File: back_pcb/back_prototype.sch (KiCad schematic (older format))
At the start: 66 parts, among them P5 CONN_01X04, P6 ATMEGA_HEADER, U1 PI ZERO

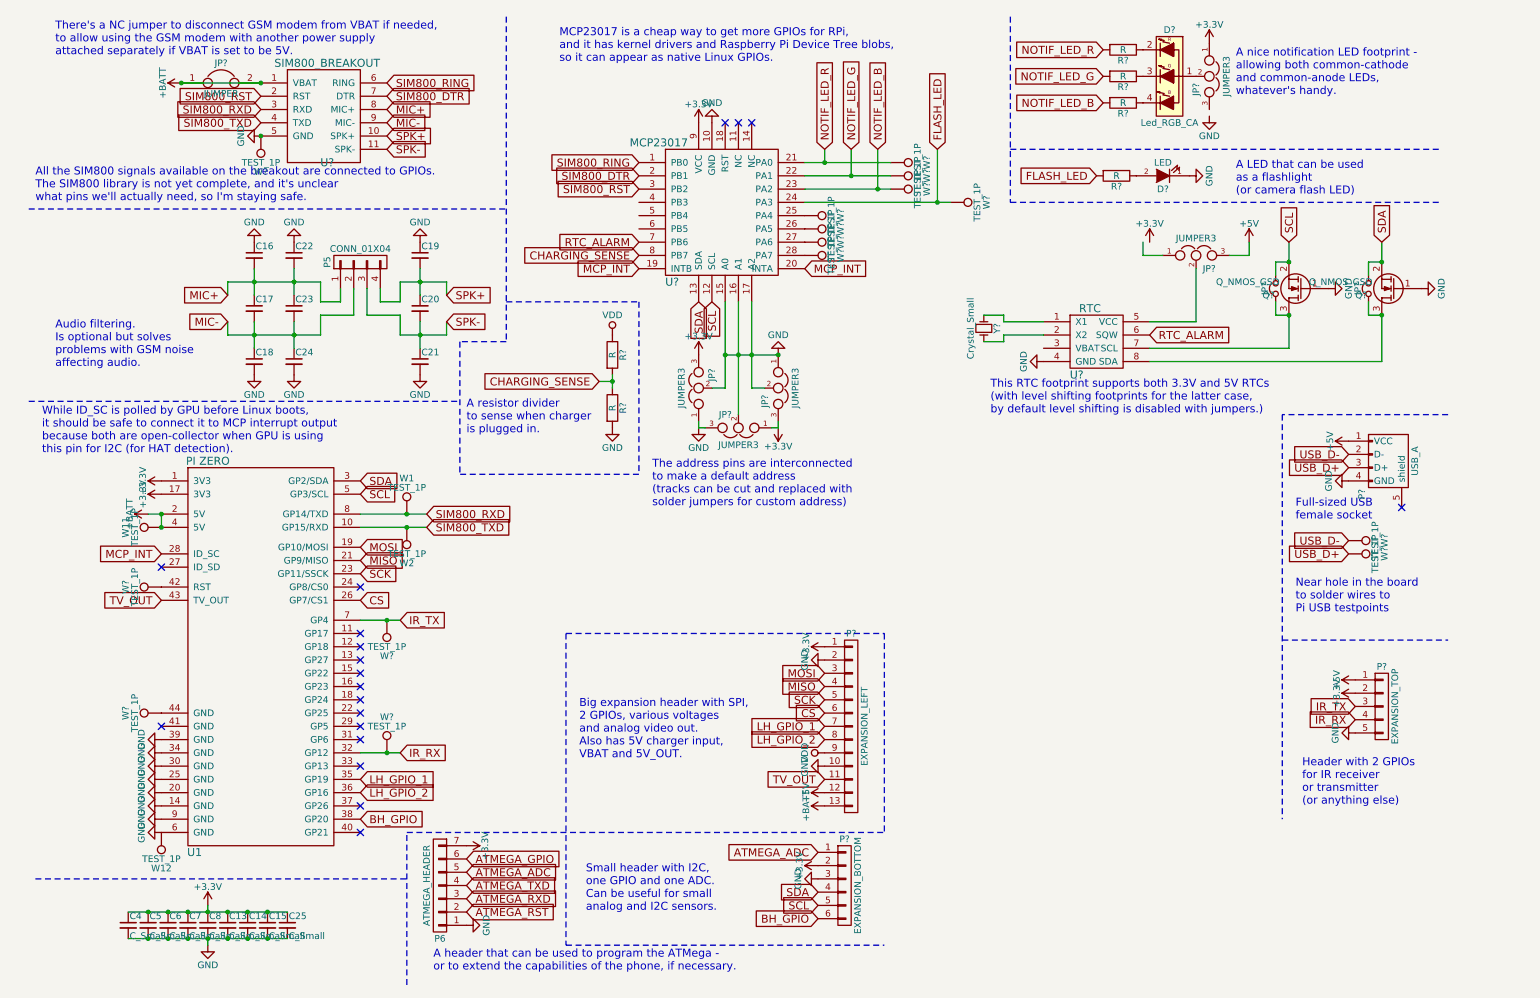
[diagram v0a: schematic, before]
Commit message: Beautiful annotations
So fabulous
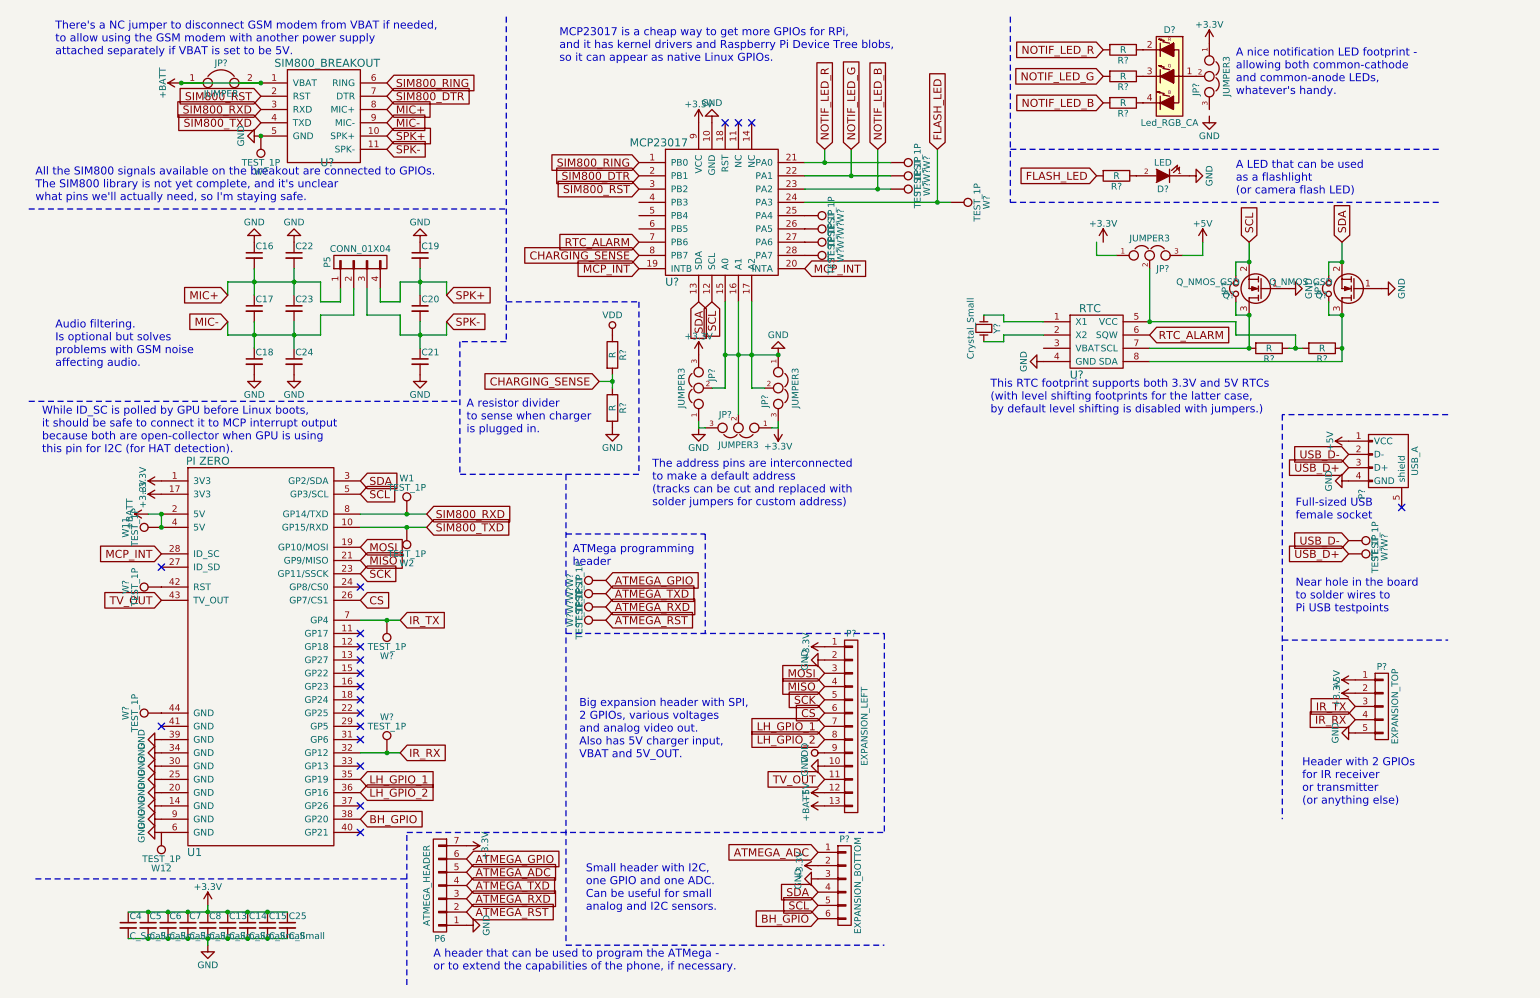
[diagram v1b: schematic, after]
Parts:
- added R? (x2): R, symbol R
- added W? (x4): TEST_1P, Measurement_Points:Measurement_Point_Square-SMD-Pad_Small, symbol TEST_1P
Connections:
- net ATMEGA_GPIO: now also W?.1
- net ATMEGA_RST: now also W?.1
- net ATMEGA_RXD: now also W?.1
- net ATMEGA_TXD: now also W?.1
- net at JP?.2, U?.5 (VCC): now also R?.1, R?.2
- net at JP?.1, Q?.3 (D), U?.7 (SCL): now also R?.2
- net at JP?.1, Q?.3 (D), U?.8 (SDA): now also R?.1
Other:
- note added: "ATMega programming \nheader"
- moved on the sheet: JP?, Q?

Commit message: Back board almost finished
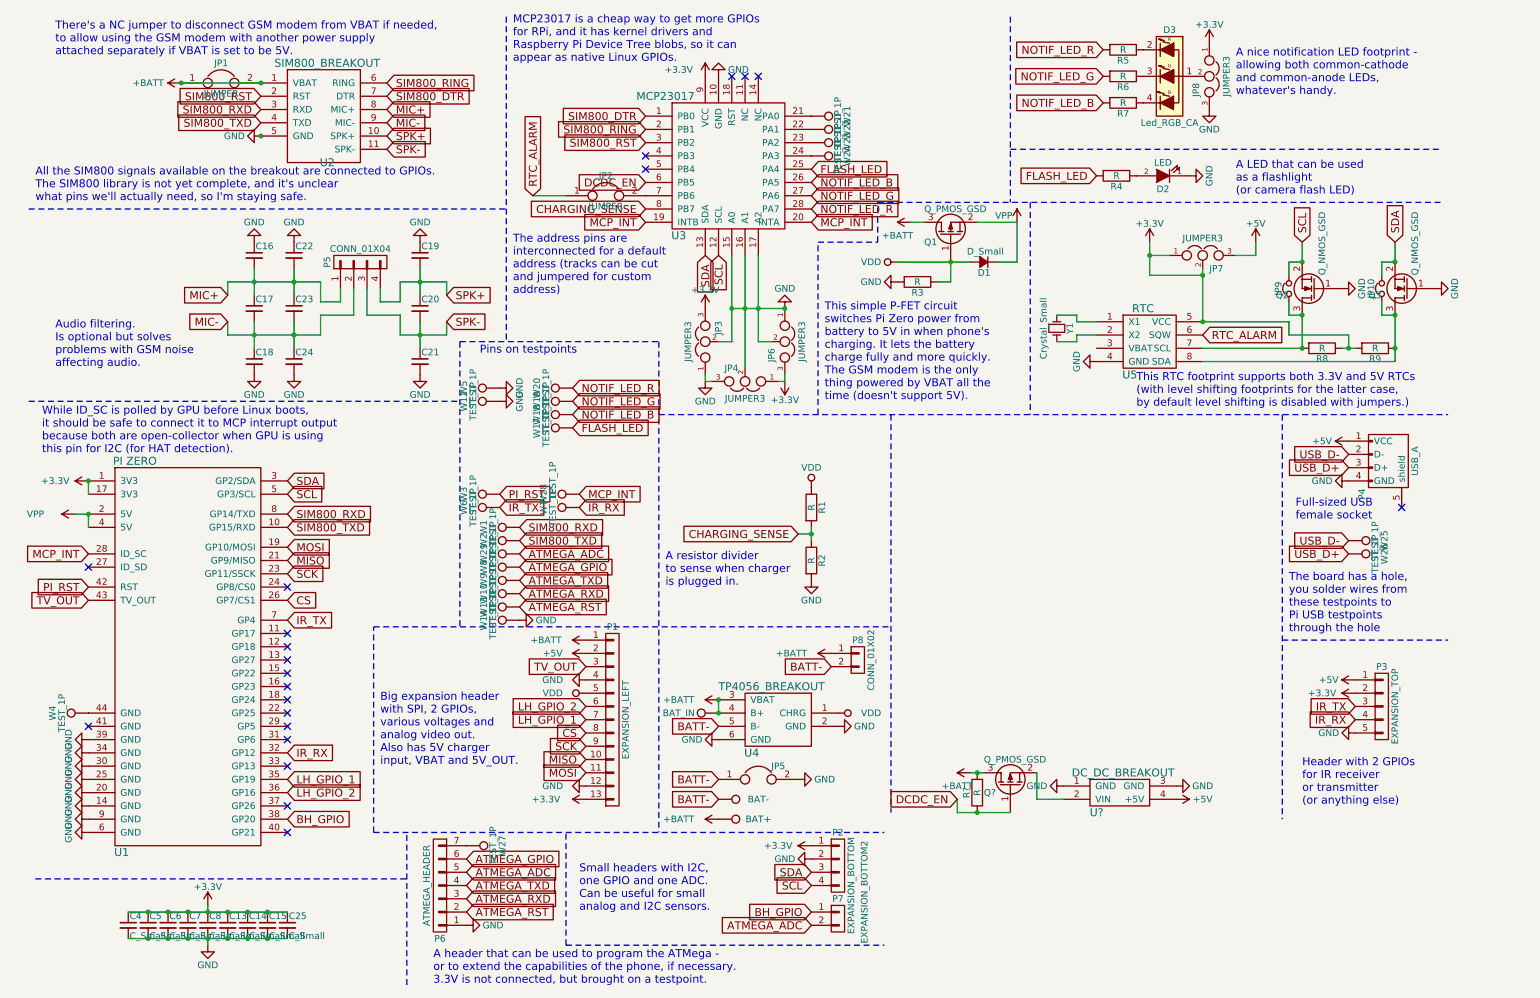
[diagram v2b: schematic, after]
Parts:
- removed P?: EXPANSION_BOTTOM, symbol CONN_01X06
- added D1: D_Small, Diodes_SMD:D_MiniMELF_Handsoldering, symbol D_Small
- added JP1, JP5: JUMPER, Connect:GS2, symbol JUMPER
- added P2: EXPANSION_BOTTOM, Pin_Headers:Pin_Header_Angled_1x04_Pitch2.54mm, symbol CONN_01X04
- added P7: EXPANSION_BOTTOM2, Pin_Headers:Pin_Header_Angled_1x02_Pitch2.54mm, symbol CONN_01X02
- added P8: CONN_01X02, footprints:JST_PH_S2B-PH-SM4-TB_02x2.00mm_Angled, symbol CONN_01X02
- added Q1, Q?: Q_PMOS_GSD, TO_SOT_Packages_SMD:SOT-23_Handsoldering, symbol Q_PMOS_GSD
- added R3, R?: R, Resistors_SMD:R_0805_HandSoldering, symbol R
- added U4: TP4056_BREAKOUT, footprints:TP4056_BREAKOUT, symbol TP4056_BREAKOUT
- added U?: DC_DC_BREAKOUT, symbol DC_DC_BREAKOUT
- added W14, W27, W28, W29: TEST_1P, Measurement_Points:Measurement_Point_Square-SMD-Pad_Small, symbol TEST_1P
- added W15: BAT-, Measurement_Points:Measurement_Point_Square-SMD-Pad_Small, symbol TEST_1P
- added W16: BAT+, Measurement_Points:Measurement_Point_Square-SMD-Pad_Small, symbol TEST_1P
- JP10, JP2, JP9: renamed from JP?; footprint (none) -> Connect:GS2
- JP3, JP4, JP6, JP7, JP8: renamed from JP?; footprint (none) -> Connect:GS3
- P1: renamed from P?; footprint (none) -> Pin_Headers:Pin_Header_Angled_1x13_Pitch2.54mm
- P3: renamed from P?; footprint (none) -> Pin_Headers:Pin_Header_Angled_1x05_Pitch2.54mm
- P4: renamed from P?; footprint (none) -> Connect:USB_A
- Q2, Q3: renamed from Q?; footprint (none) -> TO_SOT_Packages_SMD:SOT-23_Handsoldering
- R1, R2, R4, R5, R6, R7, R8, R9: renamed from R?; footprint (none) -> Resistors_SMD:R_0805_HandSoldering
- U2: renamed from U?; footprint (none) -> footprints:SIM800_BREAKOUT
- U3: renamed from U?; footprint (none) -> SMD_Packages:SOIC-28
- U5: renamed from U?; footprint (none) -> Housings_SOIC:SOIC-8_3.9x4.9mm_Pitch1.27mm
- W11: value TEST_1P -> BAT_IN
- Y1: renamed from Y?; footprint (none) -> Crystals:Crystal_SMD_G8-2pin_3.2x1.5mm_HandSoldering
- gave numbers to parts that had none: 21
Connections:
- net +3V3: now also JP7.1, JP7.2, P1.13 (P13), R8.1, R9.2, U5.5 (VCC), P2.1 (P1); no longer P1.1 (P1), P6.7 (P7)
- net +5V: now also P1.2 (P2), U?.4 (+5V); no longer P1.12 (P12)
- net +BATT: now also P1.1 (P1), JP1.1, JP1.2, P8.1 (P1), Q1.3 (D), Q?.3 (D), R?.2, U4.3 (VBAT), U4.4 (B+), W16.1; no longer JP2.1, JP2.2, P1.13 (P13), U1.2 (5V), U1.4 (5V)
- net ATMEGA_ADC: now also P7.2 (P2), W29.1
- net BH_GPIO: now also P7.1 (P1)
- net CS: now also P1.8 (P8); no longer P1.6 (P6)
- net FLASH_LED: now also U3.25 (PA4), W17.1; no longer U3.24 (PA3), W24.1
- net GND: now also JP8.3, P1.12 (P12), P1.4 (P4), JP5.2, P2.2 (P2), R3.2, U4.2 (GND), U4.6 (GND), U?.1 (GND), U?.3 (GND), W14.1; no longer P1.10 (P10), P1.2 (P2)
- net LH_GPIO_2: now also P1.6 (P6); no longer P1.8 (P8)
- net MCP_INT: now also W28.1
- net MISO: now also P1.10 (P10); no longer P1.4 (P4)
- net MOSI: now also P1.11 (P11); no longer P1.3 (P3)
- net NOTIF_LED_B: now also U3.26 (PA5), W18.1; no longer U3.23 (PA2), W23.1
- net NOTIF_LED_G: now also U3.27 (PA6), W19.1; no longer U3.22 (PA1), W22.1
- net NOTIF_LED_R: now also U3.28 (PA7), W20.1; no longer U3.21 (PA0), W21.1
- net RTC_ALARM: now also JP2.1; no longer U3.7 (PB6)
- net SCK: now also P1.9 (P9); no longer P1.5 (P5)
- net SCL: now also P2.4 (P4)
- net SDA: now also P2.3 (P3)
- net SIM800_DTR: now also U3.1 (PB0); no longer U3.2 (PB1)
- net SIM800_RING: now also U3.2 (PB1); no longer U3.1 (PB0)
- net TV_OUT: now also P1.3 (P3); no longer P1.11 (P11)
- net VDD: now also P1.5 (P5), D1.2 (A), Q1.1 (G), R3.1, U4.1 (CHRG); no longer P1.9 (P9)
- net PI_RST: now reaches U1.42 (RST), W3.1
- net DCDC_EN: now reaches U3.6 (PB5)
- net DCDC_EN: now also Q?.1 (G), R?.1
- new net: P6.7 (P7), W27.1
- new net: U3.21 (PA0), W21.1
- new net: U3.22 (PA1), W22.1
- new net: U3.23 (PA2), W23.1
- new net: U3.24 (PA3), W24.1
- new net: JP2.2, U3.7 (PB6)
- new net: Q?.2 (S), U?.2 (VIN)
- new net BATT-: JP5.1, P8.2 (P2), U4.5 (B-), W15.1
- new net VPP: D1.1 (K), Q1.2 (S), U1.2 (5V), U1.4 (5V)
- no-connect marks 19 -> 21
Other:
- note added: "A header that can be used to program the ATMega - \nor to extend the capabilities of the phone, if necessary.\n3.3V is not connected, but brought on a testpoint."
- note added: "Big expansion header \nwith SPI, 2 GPIOs, \nvarious voltages and \nanalog video out.\nAlso has 5V charger \ninput, VBAT and 5V_OUT."
- note added: "MCP23017 is a cheap way to get more GPIOs \nfor RPi, and it has kernel drivers and \nRaspberry Pi Device Tree blobs, so it can \nappear as native Linux GPIOs."
- note added: "Pins on testpoints"
- note added: "Small headers with I2C, \none GPIO and one ADC. \nCan be useful for small \nanalog and I2C sensors."
- note added: "The address pins are \ninterconnected for a default \naddress (tracks can be cut \nand jumpered for custom \naddress)"
- note added: "The board has a hole,\nyou solder wires from\nthese testpoints to\nPi USB testpoints\nthrough the hole"
- note added: "This simple P-FET circuit \nswitches Pi Zero power from \nbattery to 5V in when phone's \ncharging. It lets the battery\ncharge fully and more quickly. \nThe GSM modem is the only \nthing powered by VBAT all the \ntime (doesn't support 5V)."
- note removed: "A header that can be used to program the ATMega - \nor to extend the capabilities of the phone, if necessary."
- note removed: "ATMega programming \nheader"
- note removed: "Big expansion header with SPI,\n2 GPIOs, various voltages\nand analog video out.\nAlso has 5V charger input,\nVBAT and 5V_OUT."
- note removed: "MCP23017 is a cheap way to get more GPIOs for RPi,\nand it has kernel drivers and Raspberry Pi Device Tree blobs,\nso it can appear as native Linux GPIOs."
- note removed: "Near hole in the board\nto solder wires to \nPi USB testpoints"
- note removed: "Small header with I2C, \none GPIO and one ADC. \nCan be useful for small \nanalog and I2C sensors."
- note removed: "The address pins are interconnected\nto make a default address \n(tracks can be cut and replaced with\nsolder jumpers for custom address)"
- moved on the sheet: JP10, JP2, JP3, JP4, JP6, JP7, JP9, P1, Q2, Q3, R1, R2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
